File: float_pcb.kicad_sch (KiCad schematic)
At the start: 67 parts, among them J1 Switch, J2 Conn_01x04, J3 USB_C, J4 Conn_01x03, J5 I2C, J6 Light, J7 Batt, J9 I2C, Q1 AO3400A, Q2 AO3400A, U1 TPSM863252, U2 TPSM863252, U3 USBLC6-2SC6, U4 ESP32-S3-WROOM-1, U5 USBLC6-4SC6, U6 USBLC6-4SC6

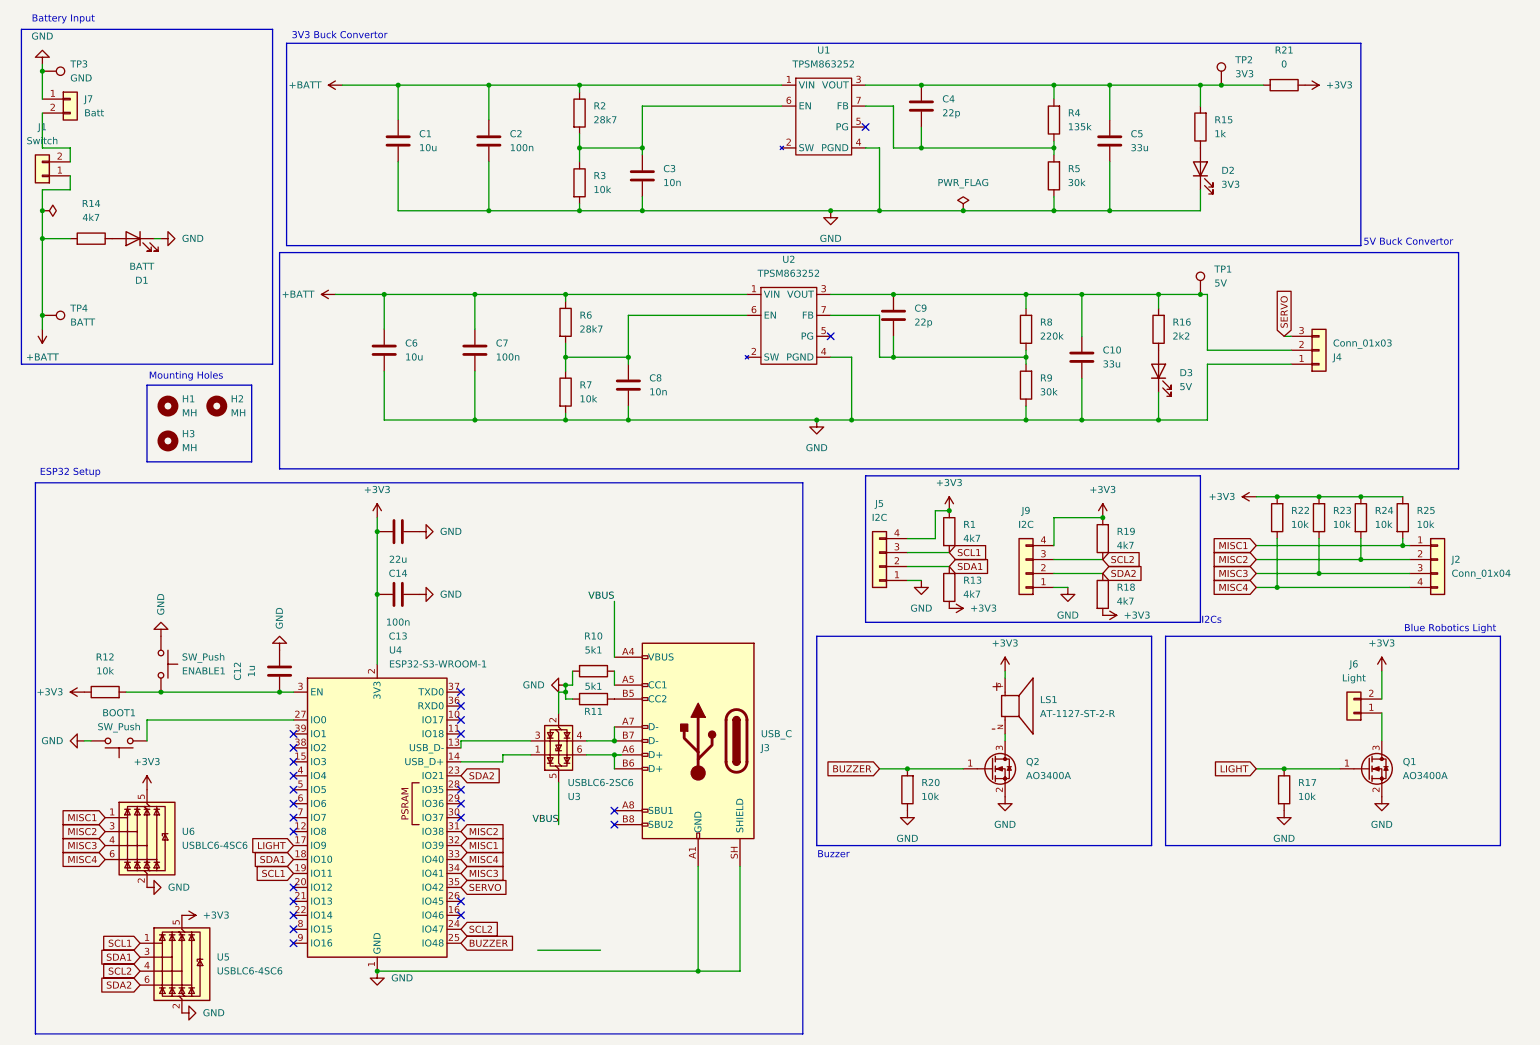
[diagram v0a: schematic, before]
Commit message: Progress
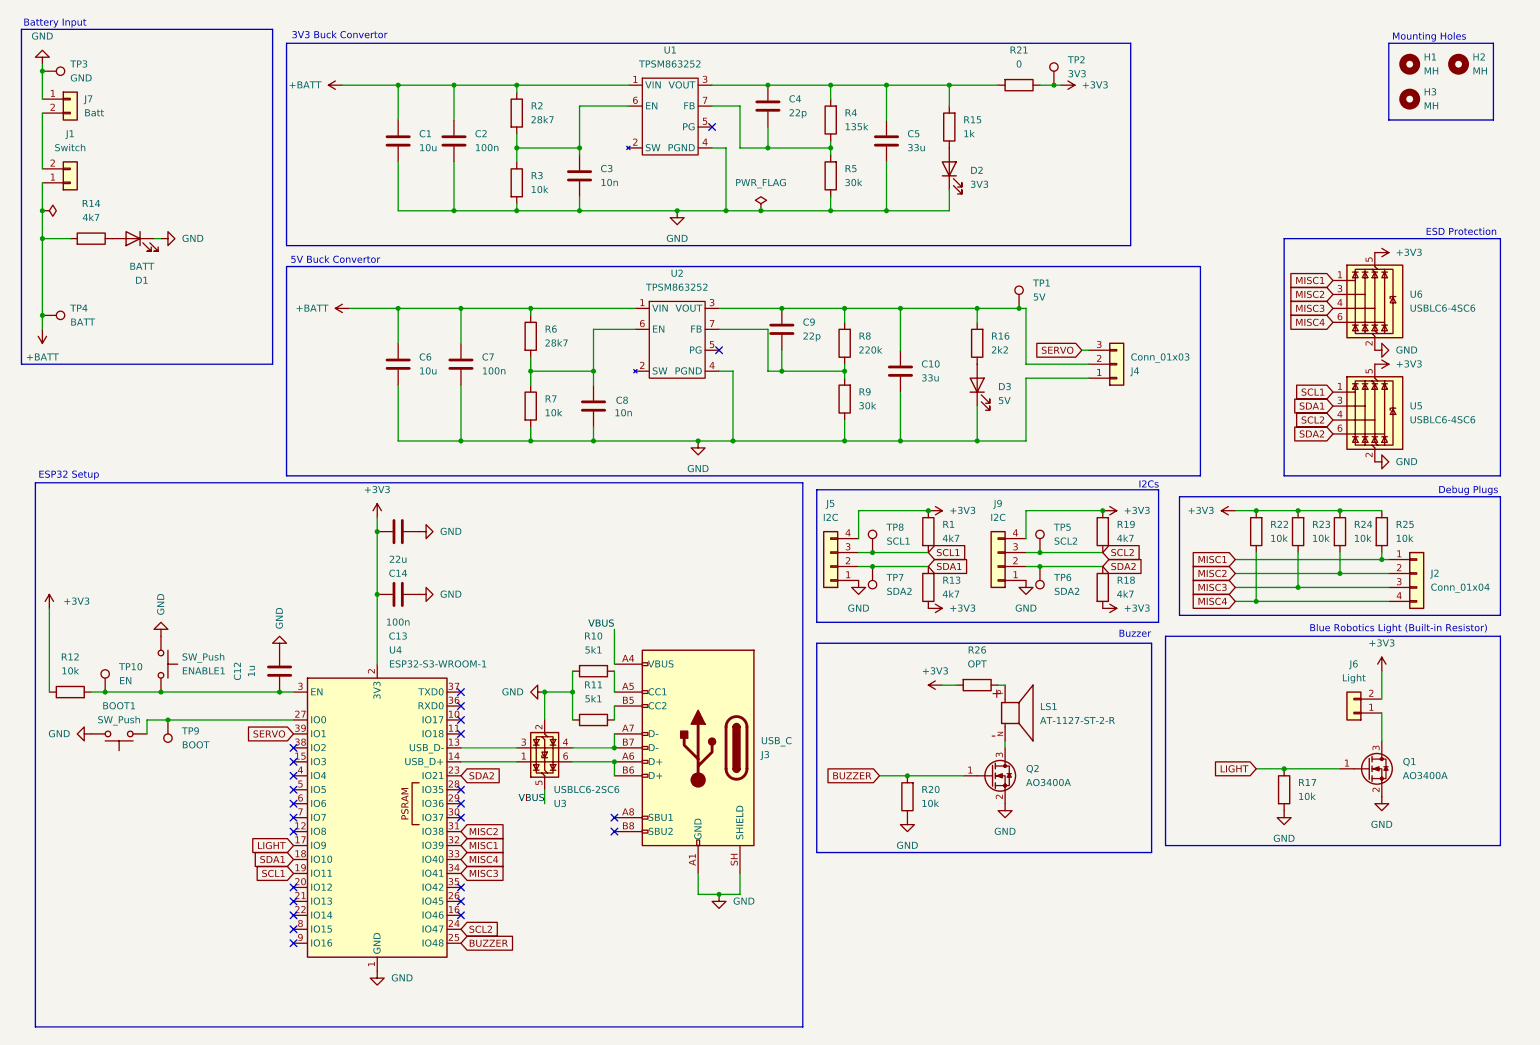
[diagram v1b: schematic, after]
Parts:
- added R26: OPT, Resistor_SMD:R_0603_1608Metric, symbol Device:R
- added TP10: EN, TestPoint:TestPoint_Pad_D1.5mm, symbol Connector:TestPoint
- added TP5: SCL2, TestPoint:TestPoint_Pad_D1.5mm, symbol Connector:TestPoint
- added TP6, TP7: SDA2, TestPoint:TestPoint_Pad_D1.5mm, symbol Connector:TestPoint
- added TP8: SCL1, TestPoint:TestPoint_Pad_D1.5mm, symbol Connector:TestPoint
- added TP9: BOOT, TestPoint:TestPoint_Pad_D1.5mm, symbol Connector:TestPoint
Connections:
- net +3V3: now also TP2.1, R26.2; no longer LS1.P
- net SCL1: now also TP8.1
- net SCL2: now also TP5.1
- net SDA1: now also TP7.1
- net SDA2: now also TP6.1
- net SERVO: now also U4.39 (IO1); no longer U4.35 (IO42)
- net at C4.1, C5.2, R15.2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: no longer TP2.1
- net at C12.2, ENABLE1.2, R12.2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: now also TP10.1
- net at BOOT1.1, U4.27 (IO0): now also TP9.1
- new net: LS1.P, R26.1
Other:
- note added: "Blue Robotics Light (Built-in Resistor)"
- note added: "Debug Plugs"
- note added: "ESD Protection"
- note removed: "Blue Robotics Light"
- moved on the sheet: BOOT1, C10, C2, C3, C4, C5, C6, C7, C8, C9, D2, D3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
